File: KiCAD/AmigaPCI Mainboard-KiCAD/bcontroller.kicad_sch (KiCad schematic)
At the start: 20 parts, among them CN227 JTAG/SWD, J200 DISABLE AUTOBOOT, U6 XC95144XL-TQ144, U711 XC9572XL-VQ64

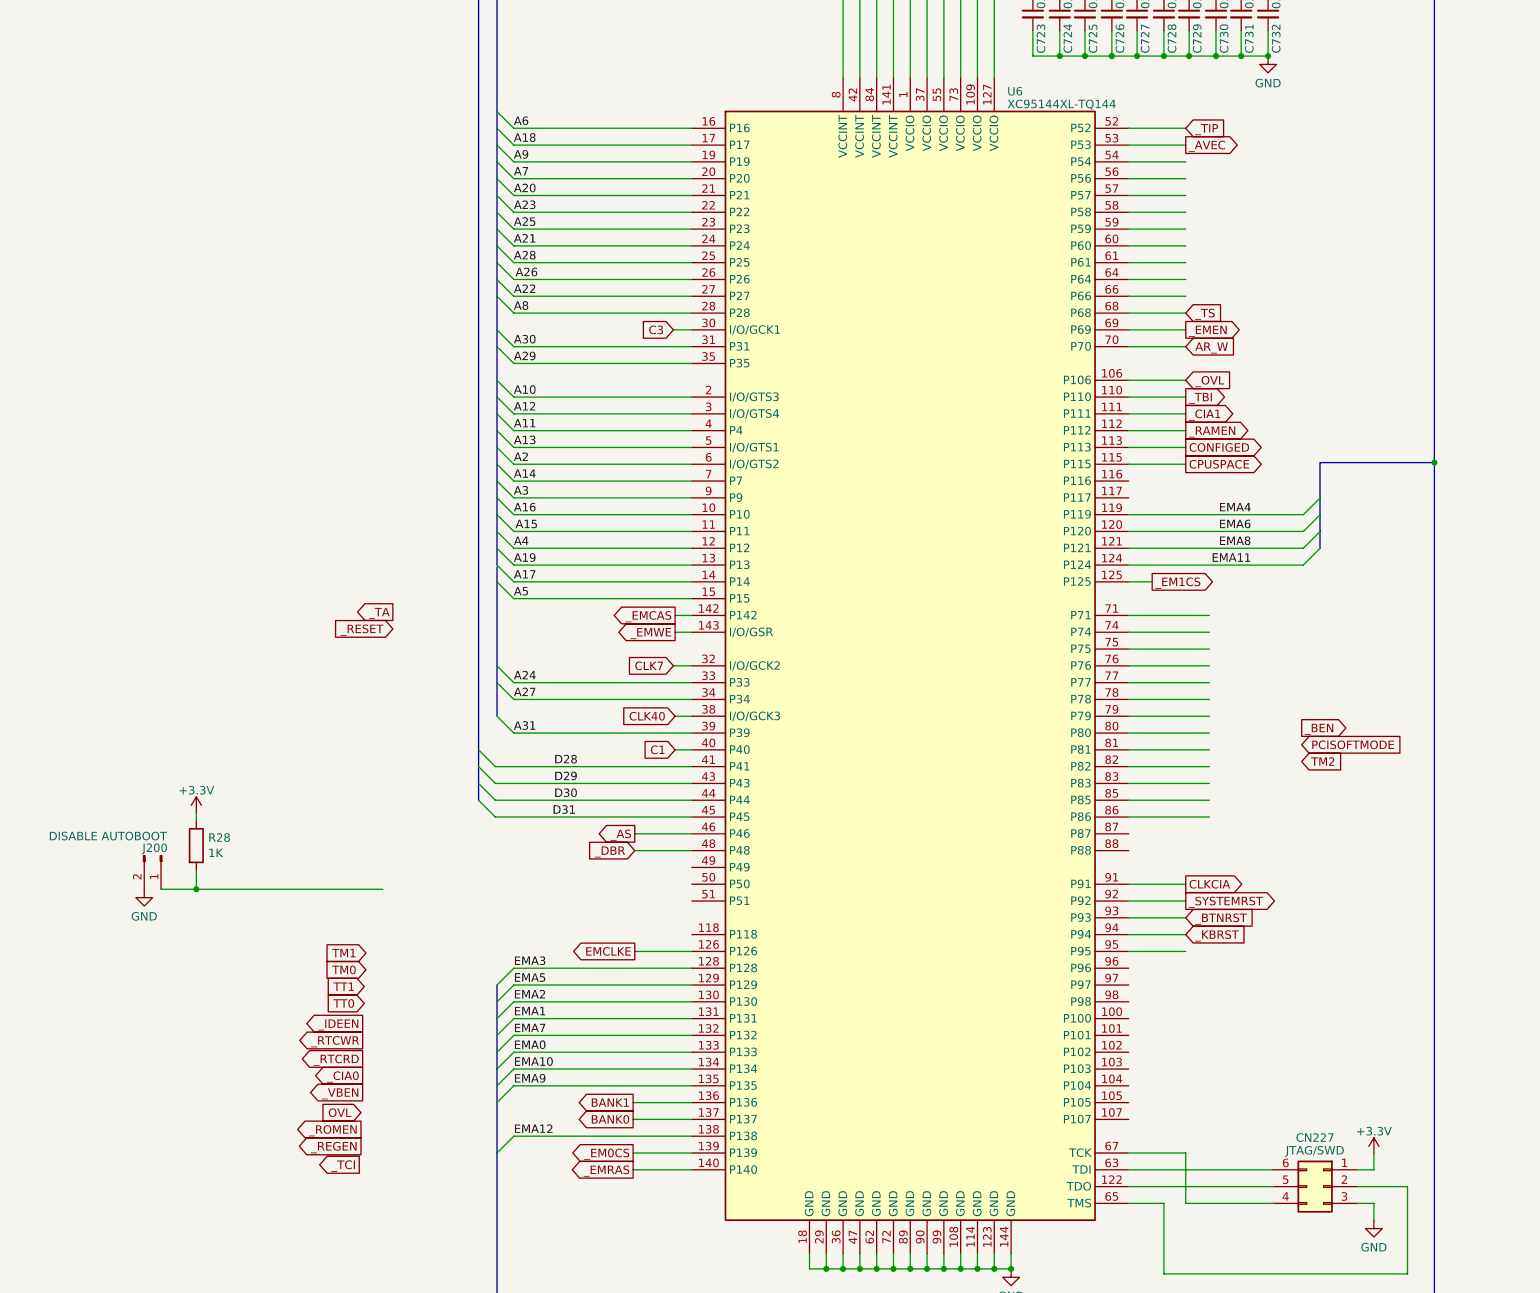
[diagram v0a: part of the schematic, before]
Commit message: Routing 17-DEC-2023
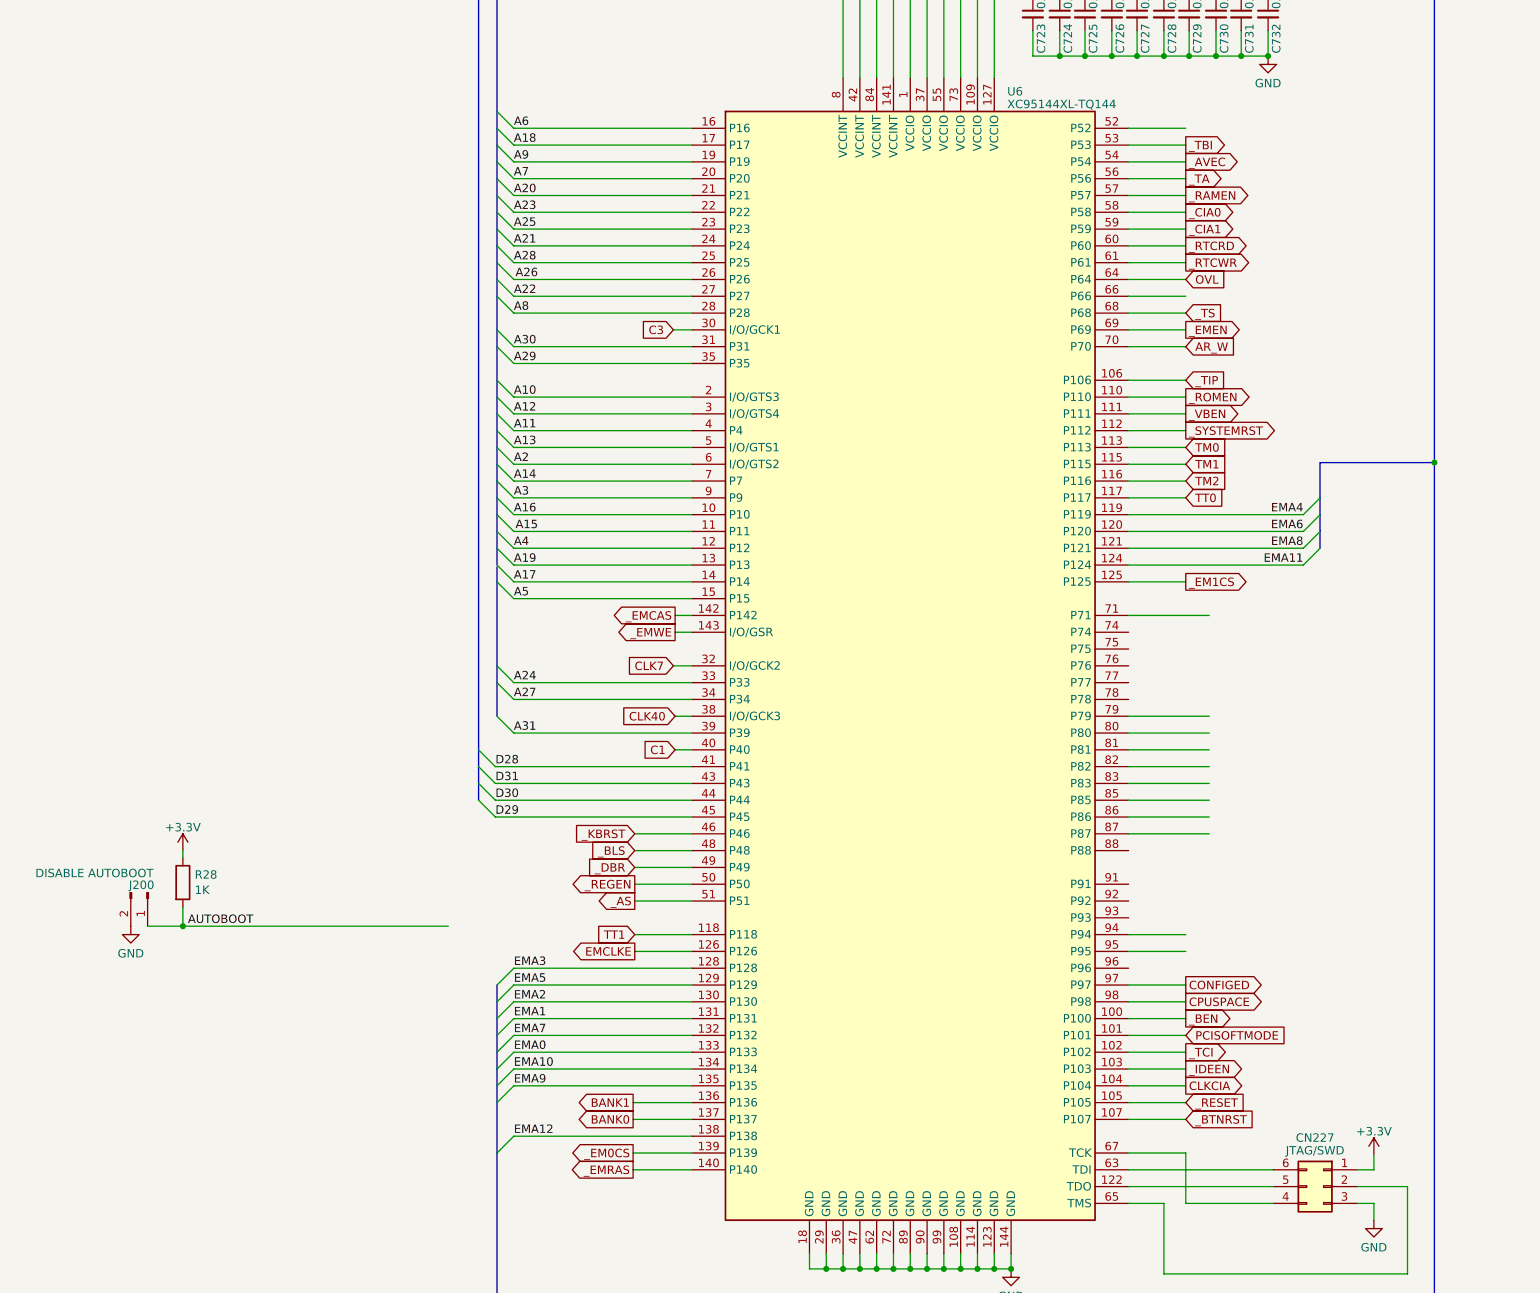
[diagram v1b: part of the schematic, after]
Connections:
- net _OVL is gone; now on net _TIP: U6.106 (P106)
- net CLKCIA: now also U6.104 (P104); no longer U6.91 (P91)
- net CONFIGED: now also U6.97 (P97); no longer U6.113 (P113)
- net CPUSPACE: now also U6.98 (P98); no longer U6.115 (P115)
- net D29: now also U6.45 (P45); no longer U6.43 (P43)
- net D31: now also U6.43 (P43); no longer U6.45 (P45)
- net OVL: now also U6.64 (P64)
- net PCISOFTMODE: now also U6.101 (P101)
- net TM0: now also U6.113 (P113)
- net TM1: now also U6.115 (P115)
- net TM2: now also U6.116 (P116)
- net TT0: now also U6.117 (P117)
- net TT1: now also U6.118 (P118)
- net _AS: now also U6.51 (P51); no longer U6.46 (P46)
- net _AVEC: now also U6.54 (P54); no longer U6.53 (P53)
- net _BEN: now also U6.100 (P100)
- net _BTNRST: now also U6.107 (P107); no longer U6.93 (P93)
- net _CIA0: now also U6.58 (P58)
- net _CIA1: now also U6.59 (P59); no longer U6.111 (P111)
- net _DBR: now also U6.49 (P49); no longer U6.48 (P48)
- net _IDEEN: now also U6.103 (P103)
- net _KBRST: now also U6.46 (P46); no longer U6.94 (P94)
- net _RAMEN: now also U6.57 (P57); no longer U6.112 (P112)
- net _REGEN: now also U6.50 (P50)
- net _RESET: now also U6.105 (P105)
- net _ROMEN: now also U6.110 (P110)
- net _RTCRD: now also U6.60 (P60)
- net _RTCWR: now also U6.61 (P61)
- net _SYSTEMRST: now also U6.112 (P112); no longer U6.92 (P92)
- net _TA: now also U6.56 (P56)
- net _TBI: now also U6.53 (P53); no longer U6.110 (P110)
- net _TCI: now also U6.102 (P102)
- net _TIP: no longer U6.52 (P52)
- net _VBEN: now also U6.111 (P111)
- net AUTOBOOT: now reaches J200.1 (Pin_1), R28.2
- new net _BLS: U6.48 (P48)
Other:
- moved on the sheet: J200, R28

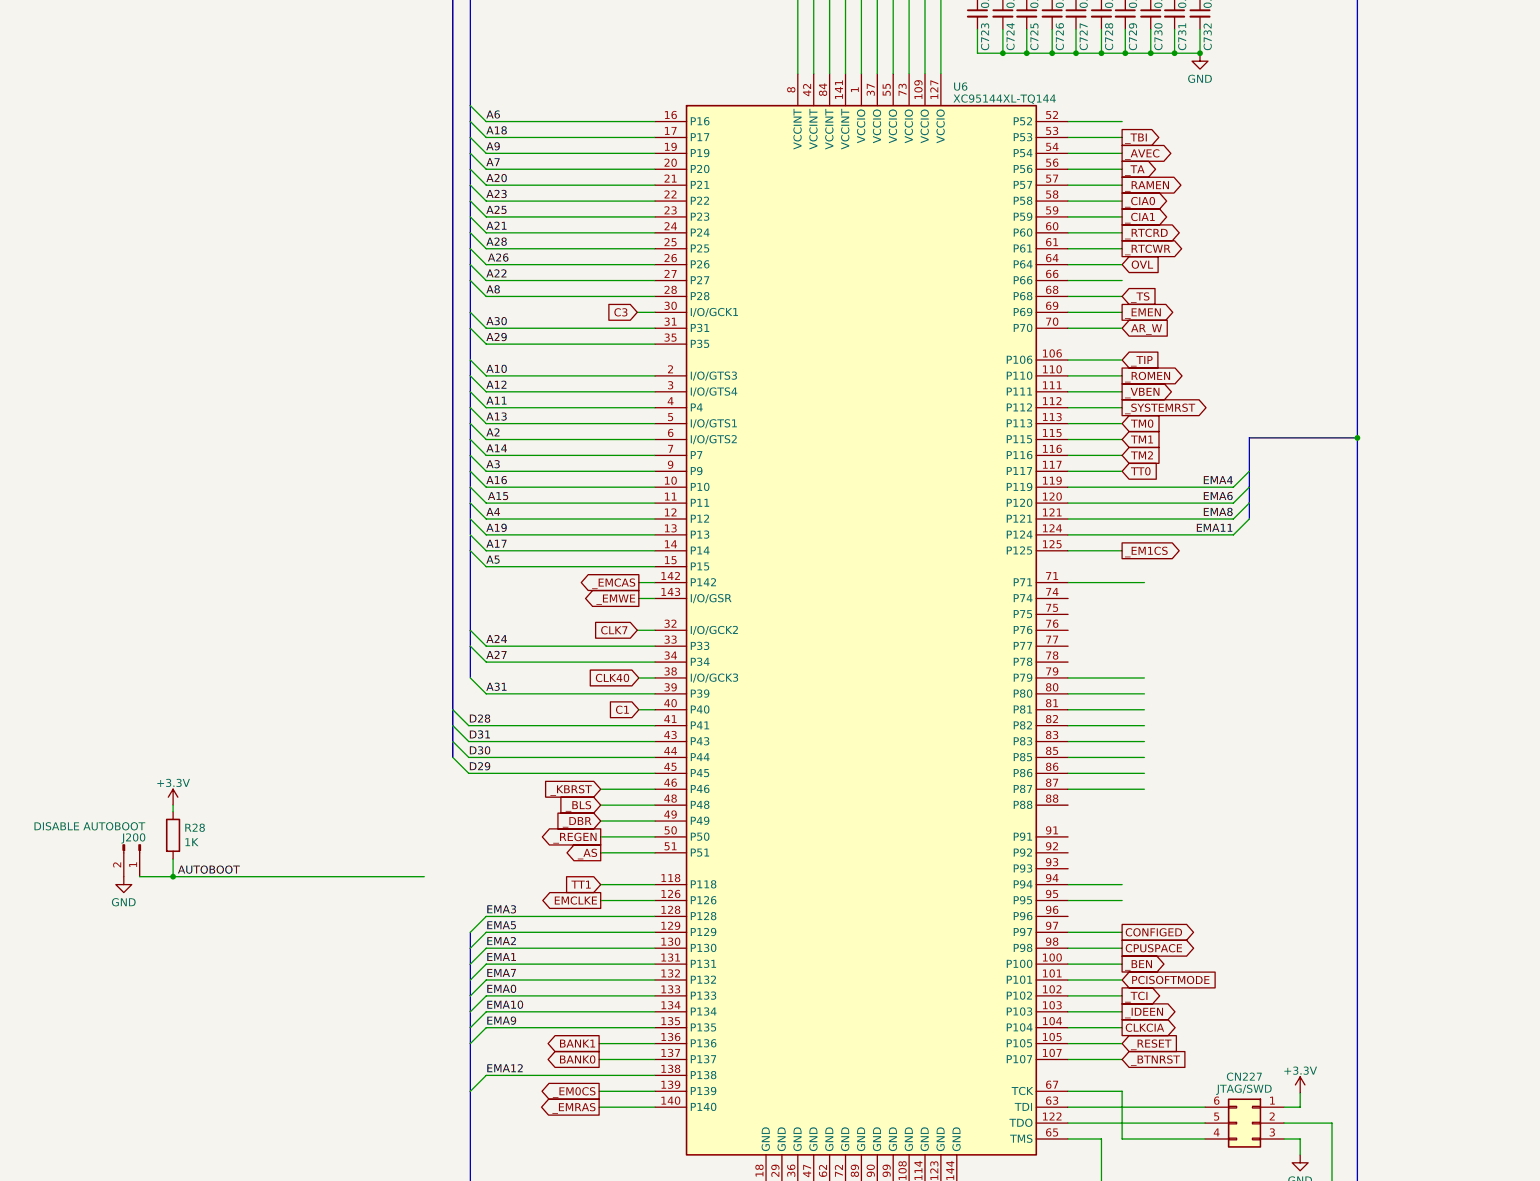
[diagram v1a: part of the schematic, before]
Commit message: Routing 18-DEC-2023
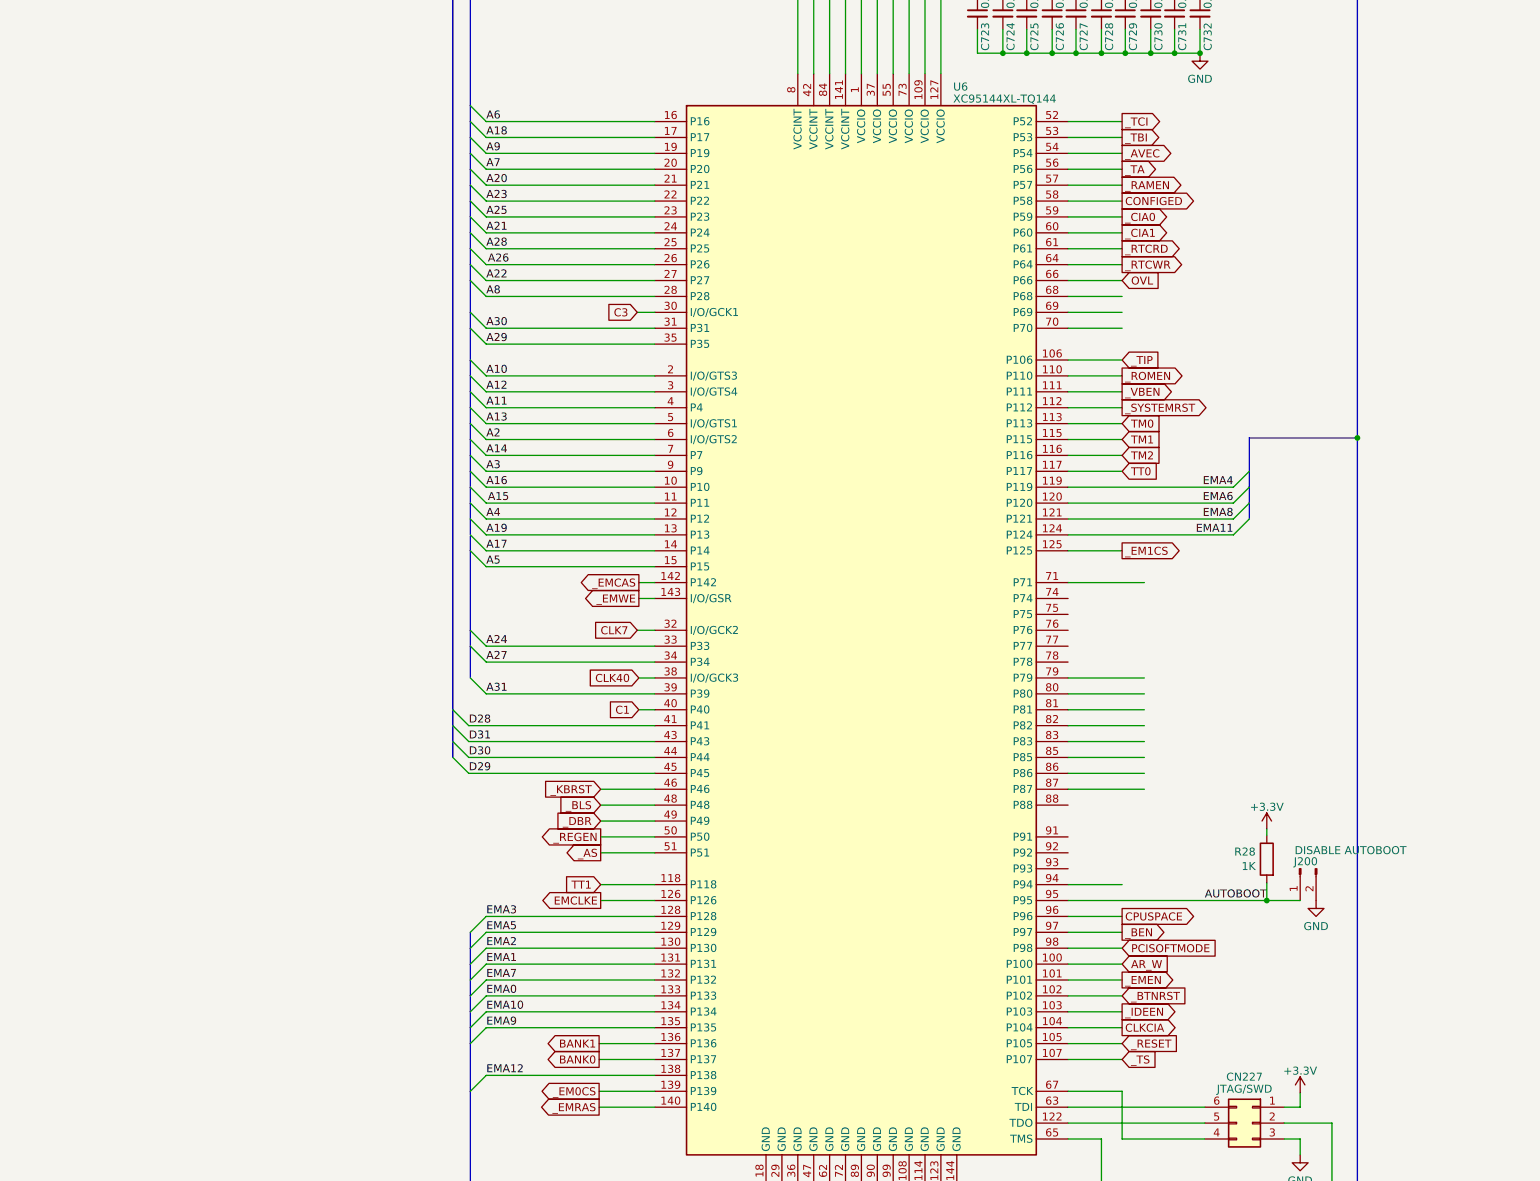
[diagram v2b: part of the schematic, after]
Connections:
- net AR_W: now also U6.100 (P100); no longer U6.70 (P70)
- net AUTOBOOT: now also U6.95 (P95)
- net CONFIGED: now also U6.58 (P58); no longer U6.97 (P97)
- net CPUSPACE: now also U6.96 (P96); no longer U6.98 (P98)
- net OVL: now also U6.66 (P66); no longer U6.64 (P64)
- net PCISOFTMODE: now also U6.98 (P98); no longer U6.101 (P101)
- net _BEN: now also U6.97 (P97); no longer U6.100 (P100)
- net _BTNRST: now also U6.102 (P102); no longer U6.107 (P107)
- net _CIA0: now also U6.59 (P59); no longer U6.58 (P58)
- net _CIA1: now also U6.60 (P60); no longer U6.59 (P59)
- net _EMEN: now also U6.101 (P101); no longer U6.69 (P69)
- net _RTCRD: now also U6.61 (P61); no longer U6.60 (P60)
- net _RTCWR: now also U6.64 (P64); no longer U6.61 (P61)
- net _TCI: now also U6.52 (P52); no longer U6.102 (P102)
- net _TS: now also U6.107 (P107); no longer U6.68 (P68)
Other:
- moved on the sheet: J200, R28
